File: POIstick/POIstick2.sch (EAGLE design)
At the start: 49 parts, among them SW1 431151015826, SW2 431151015826, U1 CR2032-SNAPDRAGONCR2032, X1 8MHz

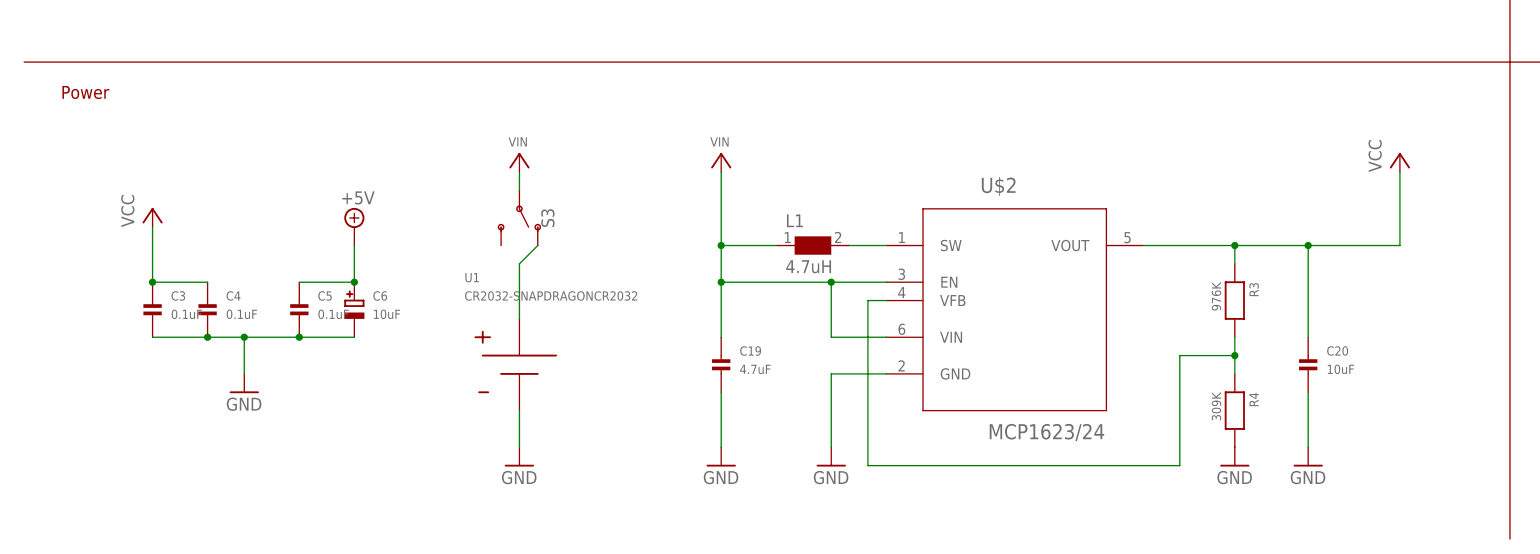
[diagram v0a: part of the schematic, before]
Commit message: WIP
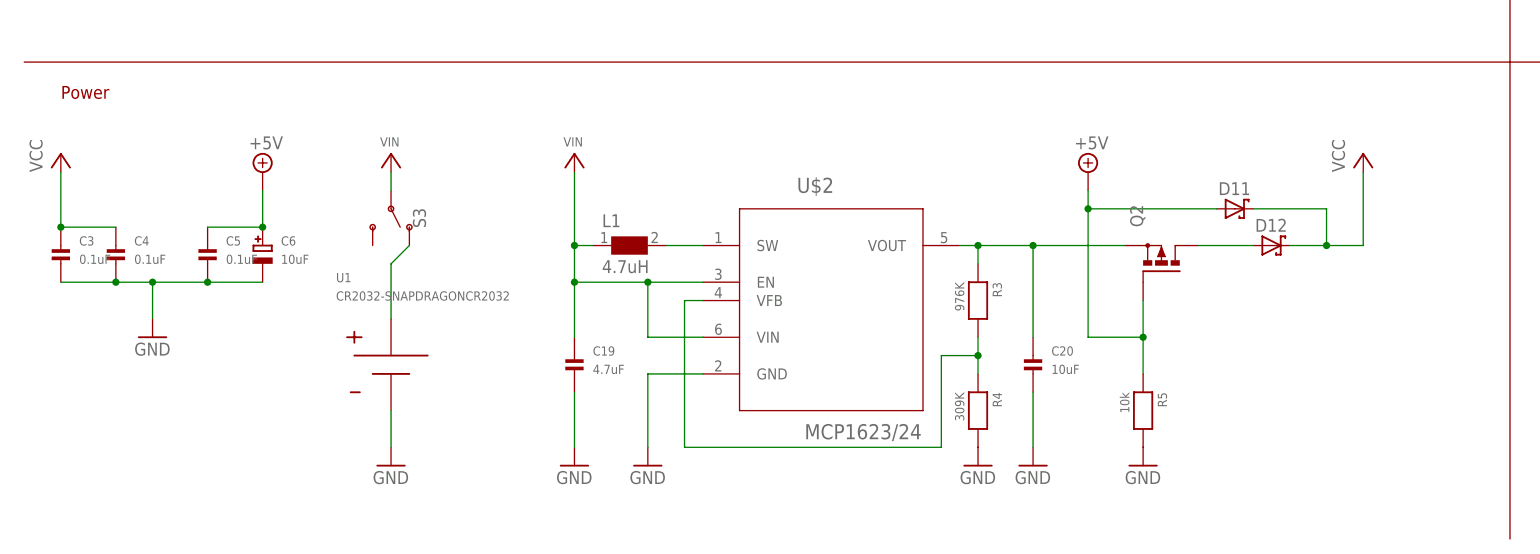
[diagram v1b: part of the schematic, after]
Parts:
- added D11, D12: (no value), eagle-ltspice:SCHOTTKY-DIODE
- added Q2: (no value), transistor-power:P-MOSFET-SO8
- added R5: 10k, microbuilder:RESISTOR0805
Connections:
- new net N$20: D12.C, Q2.D
- new net N$4: C20.P$1, Q2.S, R3.1, U$2.VOUT
- net +5V: now also D11.C, Q2.G, R5.1
- net GND: now also R5.2
- net VCC: now also D11.A, D12.A; no longer C20.P$1, R3.1, U$2.VOUT
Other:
- moved on the sheet: C19, C20, C3, C4, C5, C6, L1, R3, R4, S3, U$2, U1
